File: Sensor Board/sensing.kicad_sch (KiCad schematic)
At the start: 12 parts, among them J4 CAN Bus Connector, U4 INA180, U5 OPA323IDCKR

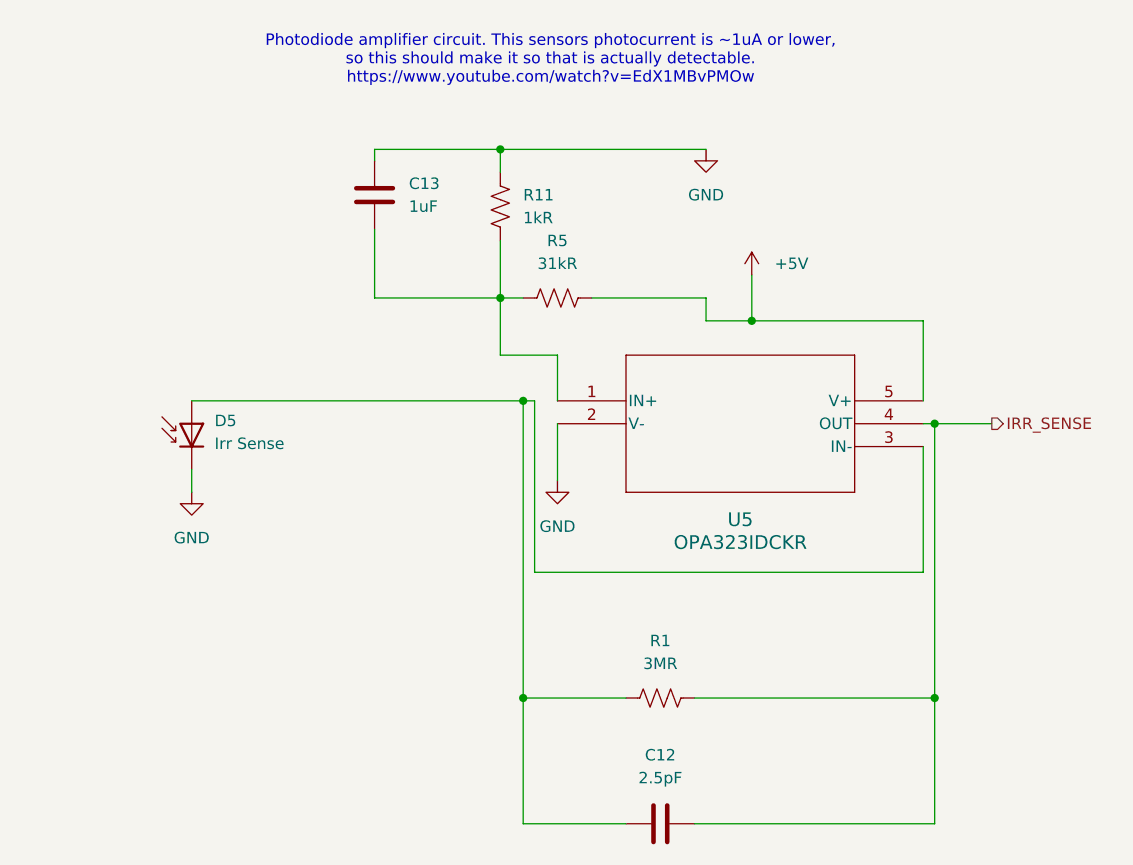
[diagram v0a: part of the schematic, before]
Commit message: Cooked another layout-Pranav
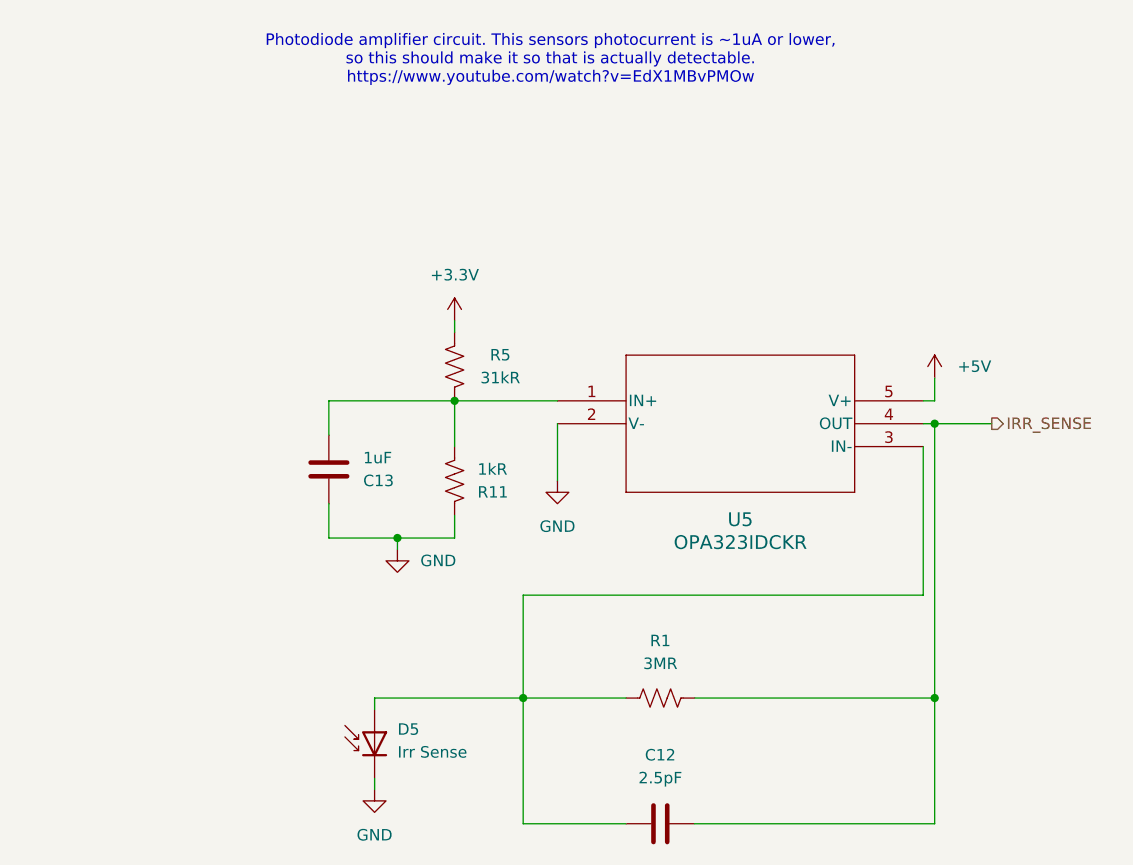
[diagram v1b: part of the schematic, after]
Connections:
- net +5V: no longer R5.2
- new net +3.3V: R5.2
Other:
- moved on the sheet: C13, D5, R11, R5

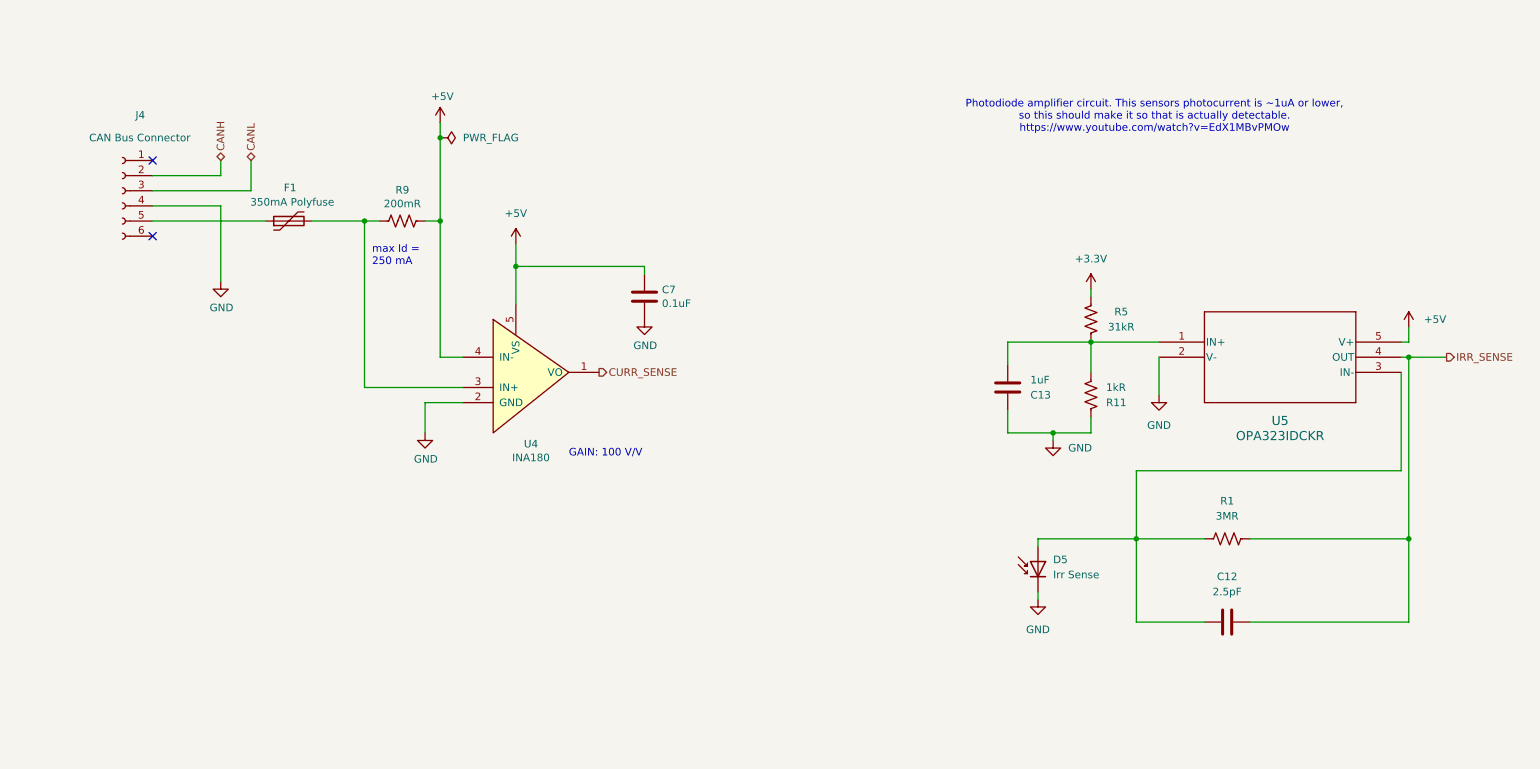
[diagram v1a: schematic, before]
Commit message: updated optics front end
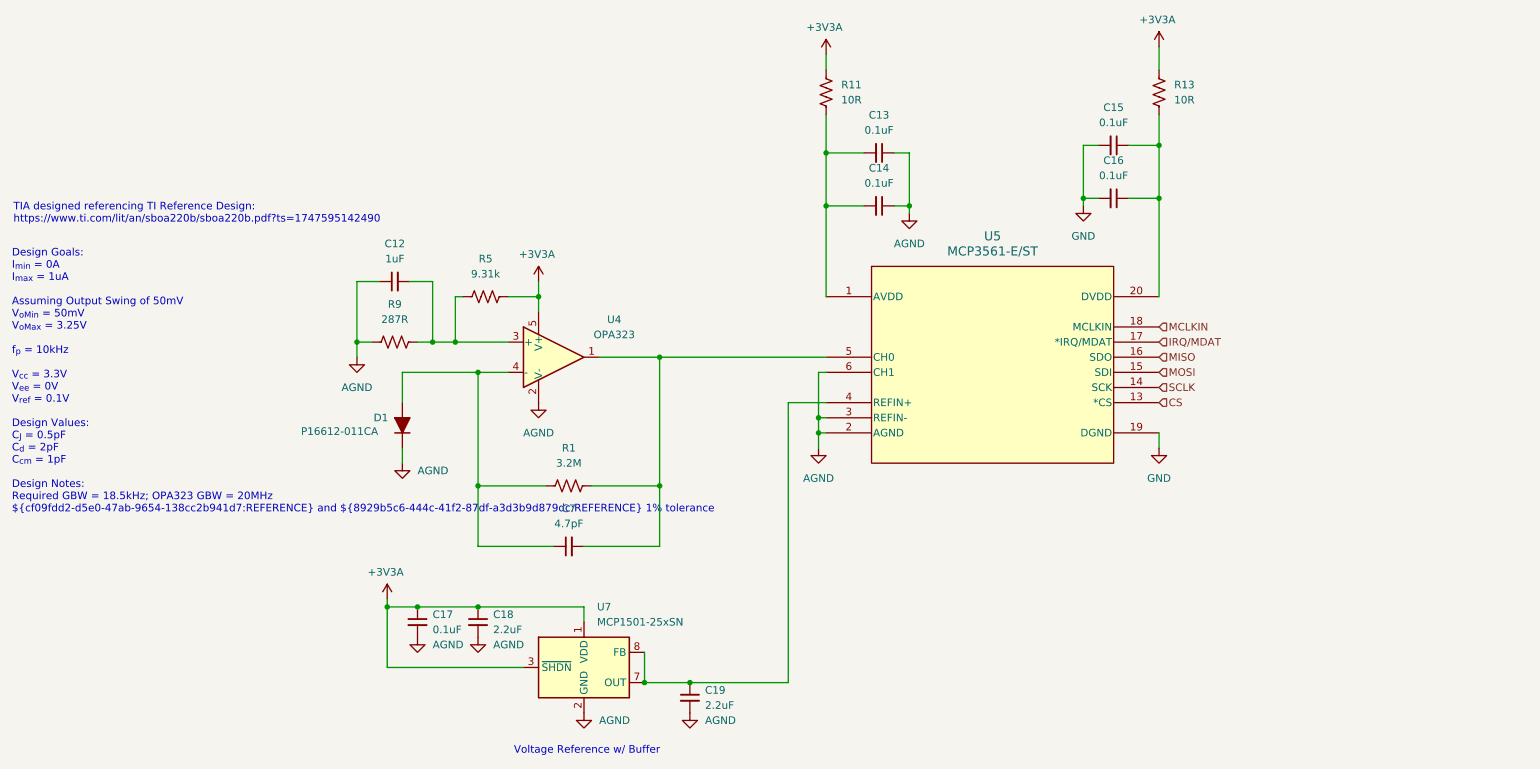
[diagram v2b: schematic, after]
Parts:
- removed C12: 2.5pF, Capacitor_SMD:C_0805_2012Metric_Pad1.18x1.45mm_HandSolder, symbol Device:C
- removed C13: 1uF, Capacitor_SMD:C_0805_2012Metric_Pad1.18x1.45mm_HandSolder, symbol Device:C
- removed C7: 0.1uF, Capacitor_SMD:C_0805_2012Metric_Pad1.18x1.45mm_HandSolder, symbol Device:C
- removed D5: Irr Sense, Canhw:P16612-011CA, symbol Device:D_Photo
- removed F1: 350mA Polyfuse, Fuse:Fuse_1206_3216Metric_Pad1.42x1.75mm_HandSolder, symbol Device:Polyfuse
- removed J4: CAN Bus Connector, Canhw:connector_Harwin_G125–MG10605M4P, symbol Connector:Conn_01x06_Socket
- removed U4: INA180, Package_TO_SOT_SMD:SOT-23-5_HandSoldering, symbol canhw:INA180
- removed U5: OPA323IDCKR, SC70-5_DCK_TEX, symbol opa323:OPA323IDCKR
- added C12: 1uF, symbol Device:C_Small
- added C13, C14, C15, C16, C17: 0.1uF, symbol Device:C_Small
- added C18, C19: 2.2uF, symbol Device:C_Small
- added C7: 4.7pF, symbol Device:C_Small
- added D1: P16612-011CA, symbol Device:D_Filled
- added R13: 10R, symbol Device:R_US
- added U4: OPA323, Package_TO_SOT_SMD:SOT-23-5, symbol Amplifier_Operational:OPA196xDBV
- added U5: MCP3561-E/ST, TSSOP20_ST_MCH, symbol PayloadSensorSymbols:MCP3561-E_ST
- added U7: MCP1501-25xSN, Package_SO:SOIC-8_3.9x4.9mm_P1.27mm, symbol Reference_Voltage:MCP1501-25xSN
- R1: value 3MR -> 3.2M; footprint Resistor_SMD:R_0805_2012Metric_Pad1.20x1.40mm_HandSolder -> (none)
- R11: value 1kR -> 10R; footprint Resistor_SMD:R_0805_2012Metric_Pad1.20x1.40mm_HandSolder -> (none)
- R5: value 31kR -> 9.31k; footprint Resistor_SMD:R_0805_2012Metric_Pad1.20x1.40mm_HandSolder -> (none)
- R9: value 200mR -> 287R; footprint Resistor_SMD:R_0805_2012Metric_Pad1.20x1.40mm_HandSolder -> (none); DigiKey WSLB-.20CT-ND -> (none)
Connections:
- net +3.3V is gone; now on an unnamed net: R5.2
- net GND: now also C15.2, C16.2, U5.11 (NC), U5.19 (DGND); no longer R11.2
- net +3V3A: now reaches R11.1, R5.1
- net +3V3A: now also C17.1, C18.1, R13.1, U4.5 (V+), U7.1 (VDD), U7.3 (~{SHDN})
- net at R1.1: now also C7.1, D1.2 (A), U4.4 (-)
- net at R9.2: now also C12.2, U4.3 (+)
- net +5V renamed AGND
- net AGND: now also C12.1, C13.1, C14.1, C17.2, C18.2, C19.2, D1.1 (K), U4.2 (V-), U5.10 (NC), U5.2 (AGND), U5.3 (REFIN-), U5.6 (CH1), U5.9 (NC), U7.2 (GND), U7.4 (GND), U7.5 (GND), U7.6 (GND)
- net IRR_SENSE: no longer names the net of R1.2
- net IRR_SENSE: now also C7.2, U4.1, U5.5 (CH0)
- new net: C13.2, C14.2, R11.2, U5.1 (AVDD)
- new net: C15.1, C16.1, R13.2, U5.20 (DVDD)
- new net: C19.1, U5.4 (REFIN+), U5.8 (NC), U7.7 (OUT), U7.8 (FB)
- new net CS: U5.13 (*CS)
- new net IRQ/MDAT: U5.17 (*IRQ/MDAT)
- new net MCLKIN: U5.18 (MCLKIN)
- new net MISO: U5.16 (SDO)
- new net MOSI: U5.15 (SDI)
- new net SCLK: U5.14 (SCK)
- no-connect marks 2 -> 0
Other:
- note added: "Design Goals: I_{min} = 0A I_{max} = 1uA Assuming Output Swing of 50mV V_{oMin} = 50mV V_{oMax} = 3.25V f_{p} = 10kHz V_{cc} = 3.3V V_{ee} = 0V V_{ref} = 0.1V Design Values: C_{J} = 0.5pF C_{d} = 2pF C_{cm} = 1pF Design Notes: Required GBW = 18.5kHz; OPA323 GBW = 20MHz ${cf09fdd2-d5e0-47ab-9654-138cc2b941d7:REFERENCE} and ${8929b5c6-444c-41f2-87df-a3d3b9d879dc:REFERENCE} 1% tolerance"
- note added: "TIA designed referencing TI Reference Design: https://www.ti.com/lit/an/sboa220b/sboa220b.pdf?ts=1747595142490"
- note added: "Voltage Reference w/ Buffer"
- note removed: "GAIN: 100 V/V"
- note removed: "Photodiode amplifier circuit. This sensors photocurrent is ~1uA or lower, so this should make it so that is actually detectable. https://www.youtube.com/watch?v=EdX1MBvPMOw"
- note removed: "max Id = 250 mA"
